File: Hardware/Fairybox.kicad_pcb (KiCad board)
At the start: 2 copper layers, 91.4 x 54.1 mm, 80 parts, among them J1 REED, J2 JST B4B-PH-K-S, Q1 locked, Q10 locked, Q14 AO3401A, Q15 SI2302, Q16 SI2302, Q2 locked, Q3 locked, Q4 locked, Q5 locked, Q6 locked, Q7 locked, Q8 locked, Q9 locked, U1 ATTINY85, U2 locked

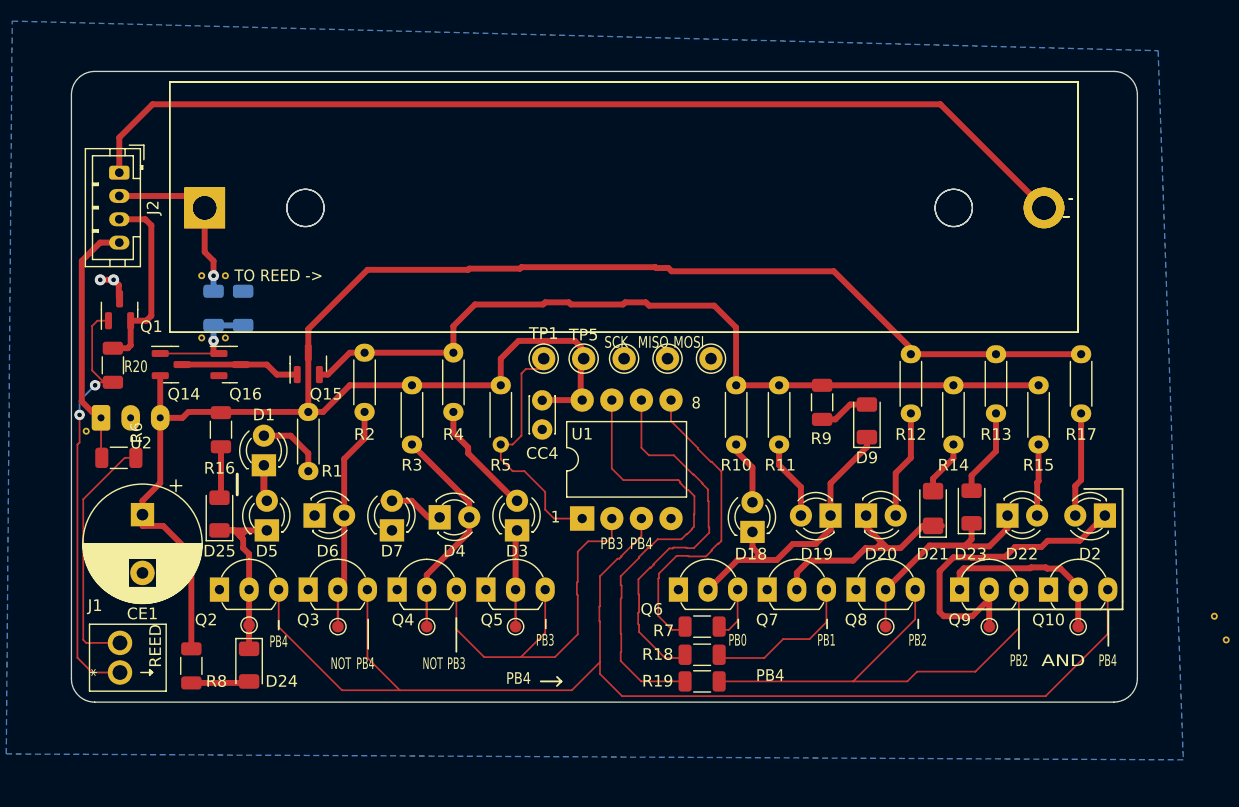
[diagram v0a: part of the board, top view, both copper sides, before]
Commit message: Edge cut.
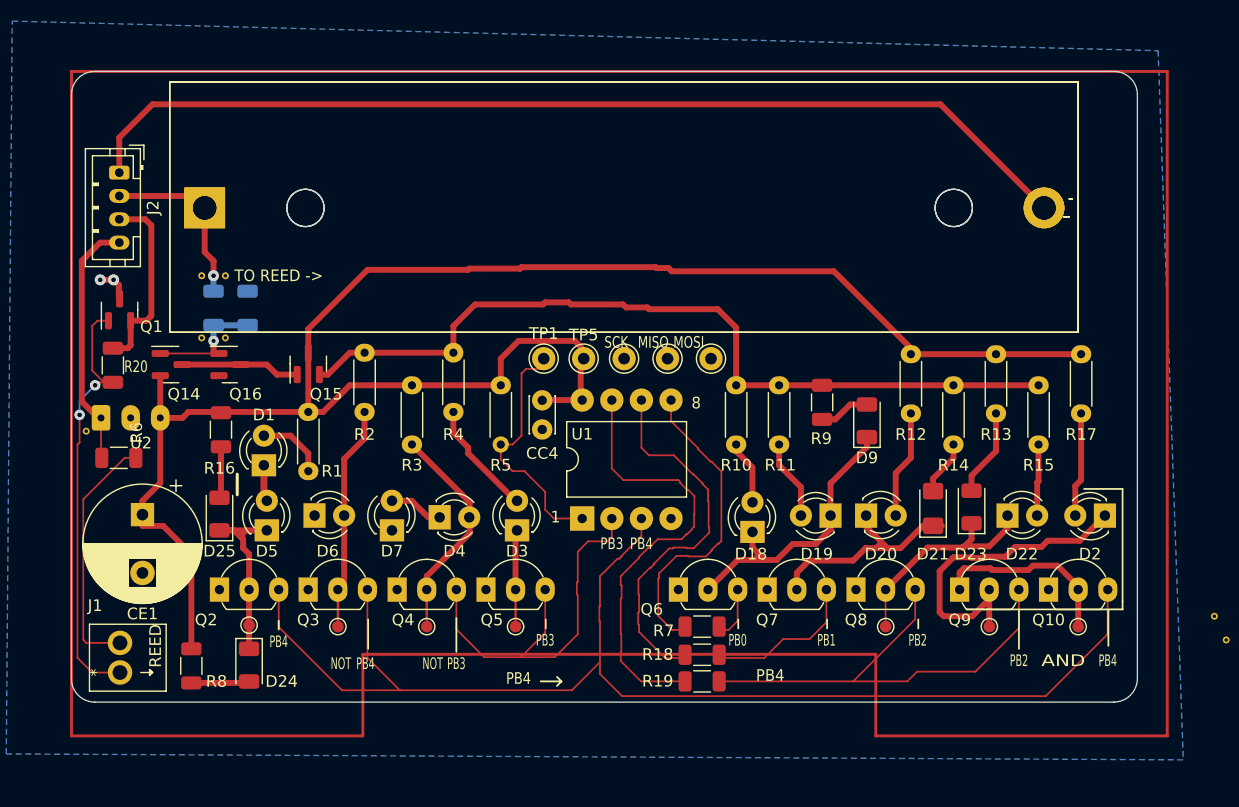
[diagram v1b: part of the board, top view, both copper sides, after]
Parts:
- moved R23 0.38 mm to (65.9, 71.1)
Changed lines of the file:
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@@
     (pad_to_mask_clearance 0)
     (solder_mask_min_width 0.12)
-    (aux_axis_origin 129.032 50.8)
+    (aux_axis_origin 50.8 50.8)
+    (grid_origin 50.8 50.8)
     (pcbplotparams
       (layerselection 0x00010fc_ffffffff)
@@
   )
   (footprint "Resistor_SMD:R_1206_3216Metric" (layer "B.Cu")
-    (at 65.532 71.12 -90)
+    (at 65.913 71.12 -90)
     (descr "Resistor SMD 1206 (3216 Metric), square (rectangular) end terminal, IPC_7351 nominal, (Body size source: IPC-SM-782 page 72, https://www.pcb-3d.com/wordpress/wp-content/uploads/ipc-sm-782a_amendment_1_and_2.pdf), generated with kicad-footprint-generator")
     (tags "resistor")
@@
     )
   )
+  (gr_line (start 119.8 107.8) (end 144.8 107.8) (layer "F.Cu") (width 0.254))
+  (gr_line (start 144.8 50.8) (end 50.8 50.8) (layer "F.Cu") (width 0.254))
+  (gr_line (start 144.8 107.8) (end 144.8 50.8) (layer "F.Cu") (width 0.254))
+  (gr_line (start 50.8 107.8) (end 75.8 107.8) (layer "F.Cu") (width 0.254))
+  (gr_line (start 75.8 107.8) (end 75.8 100.8) (layer "F.Cu") (width 0.254))
+  (gr_line (start 119.8 100.8) (end 119.8 107.8) (layer "F.Cu") (width 0.254))
+  (gr_line (start 50.8 50.8) (end 50.8 107.8) (layer "F.Cu") (width 0.254))
+  (gr_line (start 75.8 100.8) (end 119.8 100.8) (layer "F.Cu") (width 0.254))
   (gr_rect (start 121.8438 118.4148) (end 80.137 111.8108) (layer "B.SilkS") (width 0.254) (fill none))
   (gr_line (start 127.59 96.95) (end 139.07 96.95) (layer "F.SilkS") (width 0.15))
@@
   (segment (start 80.01 77.724) (end 87.63 77.724) (width 0.508) (layer "F.Cu") (net 5))
   (segment (start 93.98 73.914) (end 94.488 74.422) (width 0.508) (layer "F.Cu") (net 5))
-  (segment (start 84.92625 87.72025) (end 84.92625 90.33375) (width 0.508) (layer "F.Cu") (net 6))
   (segment (start 81.28 98.425) (end 81.28 95.25) (width 0.2) (layer "F.Cu") (net 6))
-  (segment (start 80.01 82.804) (end 84.92625 87.72025) (width 0.508) (layer "F.Cu") (net 6))
-  (segment (start 84.92625 90.33375) (end 81.28 93.98) (width 0.508) (layer "F.Cu") (net 6))
-  (segment (start 81.28 93.98) (end 81.28 95.25) (width 0.508) (layer "F.Cu") (net 6))
+  (segment (start 81.28 94.107) (end 81.28 95.25) (width 0.508) (layer "F.Cu") (net 6))
+  (segment (start 84.963 87.757) (end 84.963 90.424) (width 0.508) (layer "F.Cu") (net 6))
+  (segment (start 84.963 90.424) (end 81.28 94.107) (width 0.508) (layer "F.Cu") (net 6))
+  (segment (start 80.01 82.804) (end 84.963 87.757) (width 0.508) (layer "F.Cu") (net 6))
   (segment (start 67.31 87.63) (end 67.31 84.587) (width 0.6) (layer "F.Cu") (net 7))
   (segment (start 69.601 82.047) (end 71.12 83.566) (width 0.508) (layer "F.Cu") (net 8))
@@
   (segment (start 133.641665 86.068335) (end 133.762625 85.947375) (width 0.508) (layer "F.Cu") (net 14))
   (segment (start 131.101665 88.9) (end 131.101665 89.979935) (width 0.508) (layer "F.Cu") (net 15))
-  (segment (start 124.4246 91.4654) (end 120.64 95.25) (width 0.508) (layer "F.Cu") (net 15))
-  (segment (start 127.4826 91.4654) (end 128.016 90.932) (width 0.508) (layer "F.Cu") (net 15))
+  (segment (start 120.64 95.25) (end 124.2468 91.6432) (width 0.508) (layer "F.Cu") (net 15))
+  (segment (start 124.2468 91.6432) (end 127.3048 91.6432) (width 0.508) (layer "F.Cu") (net 15))
+  (segment (start 127.3048 91.6432) (end 128.016 90.932) (width 0.508) (layer "F.Cu") (net 15))
   (segment (start 131.101665 89.979935) (end 129.54 91.5416) (width 0.508) (layer "F.Cu") (net 15))
-  (segment (start 124.4246 91.4654) (end 127.4826 91.4654) (width 0.508) (layer "F.Cu") (net 15))
   (segment (start 129.54 91.5416) (end 127.3302 91.5416) (width 0.508) (layer "F.Cu") (net 15))
-  (segment (start 128.016 90.932) (end 128.016 89.5664) (width 0.508) (layer "F.Cu") (net 15))
   (segment (start 120.64 98.796) (end 120.64 95.25) (width 0.15) (layer "F.Cu") (net 15))
+  (segment (start 128.016 90.932) (end 128.016 89.5664) (width 0.508) (layer "F.Cu") (net 15))
   (segment (start 54.9656 99.822) (end 52.07 99.822) (width 0.1524) (layer "F.Cu") (net 16))
   (segment (start 51.816 99.568) (end 51.816 87.503) (width 0.1524) (layer "F.Cu") (net 16))
@@
   (segment (start 111.506 84.582) (end 111.506 82.804) (width 0.508) (layer "F.Cu") (net 19))
   (segment (start 113.3793 88.699967) (end 113.3793 86.4553) (width 0.508) (layer "F.Cu") (net 19))
-  (segment (start 127.3556 93.4212) (end 133.0452 93.4212) (width 0.508) (layer "F.Cu") (net 20))
-  (segment (start 134.3914 93.345) (end 134.493 93.4466) (width 0.508) (layer "F.Cu") (net 20))
-  (segment (start 135.587822 93.4466) (end 135.613222 93.4212) (width 0.508) (layer "F.Cu") (net 20))
+  (segment (start 129.794 93.5736) (end 132.8928 93.5736) (width 0.508) (layer "F.Cu") (net 20))
+  (segment (start 133.2738 93.1926) (end 135.384622 93.1926) (width 0.508) (layer "F.Cu") (net 20))
   (segment (start 137.16 95.25) (end 137.16 98.425) (width 0.508) (layer "F.Cu") (net 20))
   (segment (start 126.99 93.7868) (end 127.3556 93.4212) (width 0.508) (layer "F.Cu") (net 20))
-  (segment (start 133.1214 93.345) (end 134.3914 93.345) (width 0.508) (layer "F.Cu") (net 20))
-  (segment (start 134.493 93.4466) (end 135.587822 93.4466) (width 0.508) (layer "F.Cu") (net 20))
-  (segment (start 135.613222 93.4212) (end 137.16 94.967978) (width 0.508) (layer "F.Cu") (net 20))
+  (segment (start 132.8928 93.5736) (end 133.2738 93.1926) (width 0.508) (layer "F.Cu") (net 20))
+  (segment (start 127.3556 93.4212) (end 129.6416 93.4212) (width 0.508) (layer "F.Cu") (net 20))
+  (segment (start 135.384622 93.1926) (end 137.16 94.967978) (width 0.508) (layer "F.Cu") (net 20))
   (segment (start 126.99 95.25) (end 126.99 93.7868) (width 0.508) (layer "F.Cu") (net 20))
-  (segment (start 133.0452 93.4212) (end 133.1214 93.345) (width 0.508) (layer "F.Cu") (net 20))
+  (segment (start 129.6416 93.4212) (end 129.794 93.5736) (width 0.508) (layer "F.Cu") (net 20))
   (segment (start 83.566 81.788) (end 84.836 83.058) (width 0.508) (layer "F.Cu") (net 21))
   (segment (start 83.566 80.01) (end 83.566 81.788) (width 0.508) (layer "F.Cu") (net 21))
@@
   (segment (start 51.499661 80.264) (end 51.499661 79.056339) (width 0.1524) (layer "B.Cu") (net 40))
   (segment (start 51.499661 79.056339) (end 52.832 77.724) (width 0.1524) (layer "B.Cu") (net 40))
+  (segment (start 91.44 70.612) (end 93.472 70.612) (width 0.508) (layer "F.Cu") (net 41))
   (segment (start 107.823 77.724) (end 111.474375 77.724) (width 0.508) (layer "F.Cu") (net 41))
+  (segment (start 106.2482 71.1962) (end 107.815 72.763) (width 0.508) (layer "F.Cu") (net 41))
+  (segment (start 100.3554 71.1962) (end 106.2482 71.1962) (width 0.508) (layer "F.Cu") (net 41))
   (segment (start 93.6498 70.7898) (end 98.1202 70.7898) (width 0.508) (layer "F.Cu") (net 41))
-  (segment (start 107.815 72.763) (end 107.815 76.962) (width 0.508) (layer "F.Cu") (net 41))
-  (segment (start 91.2622 70.7898) (end 91.44 70.612) (width 0.508) (layer "F.Cu") (net 41))
   (segment (start 85.4202 70.7898) (end 91.2622 70.7898) (width 0.508) (layer "F.Cu") (net 41))
   (segment (start 93.472 70.612) (end 93.6498 70.7898) (width 0.508) (layer "F.Cu") (net 41))
-  (segment (start 100.3554 70.8914) (end 105.9434 70.8914) (width 0.508) (layer "F.Cu") (net 41))
-  (segment (start 98.298 70.612) (end 100.076 70.612) (width 0.508) (layer "F.Cu") (net 41))
-  (segment (start 105.9434 70.8914) (end 107.815 72.763) (width 0.508) (layer "F.Cu") (net 41))
-  (segment (start 98.1202 70.7898) (end 98.298 70.612) (width 0.508) (layer "F.Cu") (net 41))
   (segment (start 75.946 74.93) (end 83.566 74.93) (width 0.508) (layer "F.Cu") (net 41))
-  (segment (start 100.076 70.612) (end 100.3554 70.8914) (width 0.508) (layer "F.Cu") (net 41))
   (segment (start 74.676 74.93) (end 75.946 74.93) (width 0.508) (layer "F.Cu") (net 41))
-  (segment (start 83.566 72.644) (end 85.4202 70.7898) (width 0.508) (layer "F.Cu") (net 41))
-  (segment (start 91.44 70.612) (end 93.472 70.612) (width 0.508) (layer "F.Cu") (net 41))
+  (segment (start 83.566 74.93) (end 83.566 72.644) (width 0.508) (layer "F.Cu") (net 41))
+  (segment (start 107.815 72.763) (end 107.815 76.962) (width 0.508) (layer "F.Cu") (net 41))
   (segment (start 111.474375 77.724) (end 115.19575 77.724) (width 0.508) (layer "F.Cu") (net 41))
   (segment (start 72.801 76.805) (end 74.676 74.93) (width 0.508) (layer "F.Cu") (net 41))
+  (segment (start 91.2622 70.7898) (end 91.44 70.612) (width 0.508) (layer "F.Cu") (net 41))
+  (segment (start 83.566 72.644) (end 85.4202 70.7898) (width 0.508) (layer "F.Cu") (net 41))
   (segment (start 126.459875 77.724) (end 133.762625 77.724) (width 0.508) (layer "F.Cu") (net 41))
-  (segment (start 83.566 74.93) (end 83.566 72.644) (width 0.508) (layer "F.Cu") (net 41))
+  (segment (start 98.1202 70.7898) (end 98.3742 71.0438) (width 0.508) (layer "F.Cu") (net 41))
+  (segment (start 100.203 71.0438) (end 100.3554 71.1962) (width 0.508) (layer "F.Cu") (net 41))
   (segment (start 115.19575 77.724) (end 126.459875 77.724) (width 0.508) (layer "F.Cu") (net 41))
   (segment (start 72.07 76.805) (end 72.801 76.805) (width 0.508) (layer "F.Cu") (net 41))
+  (segment (start 98.3742 71.0438) (end 100.203 71.0438) (width 0.508) (layer "F.Cu") (net 41))
   (segment (start 58.42 74.996) (end 63.18 74.996) (width 0.1524) (layer "F.Cu") (net 42))
   (segment (start 62.992 74.996) (end 62.992 73.914) (width 0.508) (layer "F.Cu") (net 42))
